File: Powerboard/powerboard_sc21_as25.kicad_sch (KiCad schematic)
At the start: 44 parts, among them J10 Conn_01x04_Male, J2 Conn_01x02_Male, J3 Conn_01x02_Male, J4 Conn_01x08_Male, J9 Conn_Coaxial, Q6 MMDT2222A, Q7 RSJ250P10TL, Q8 RSJ250P10TL, U1 LTC4412xS6, U2 SN65HVD230, U3 ESP32-PICO-D4

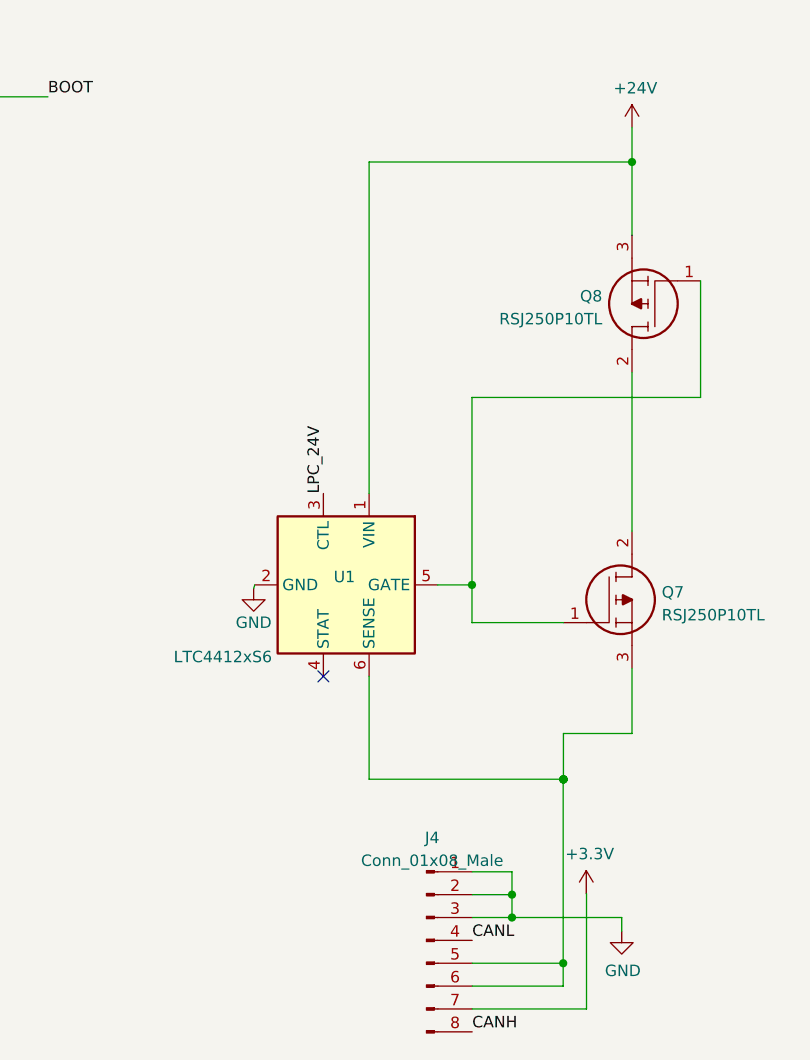
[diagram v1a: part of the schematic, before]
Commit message: update
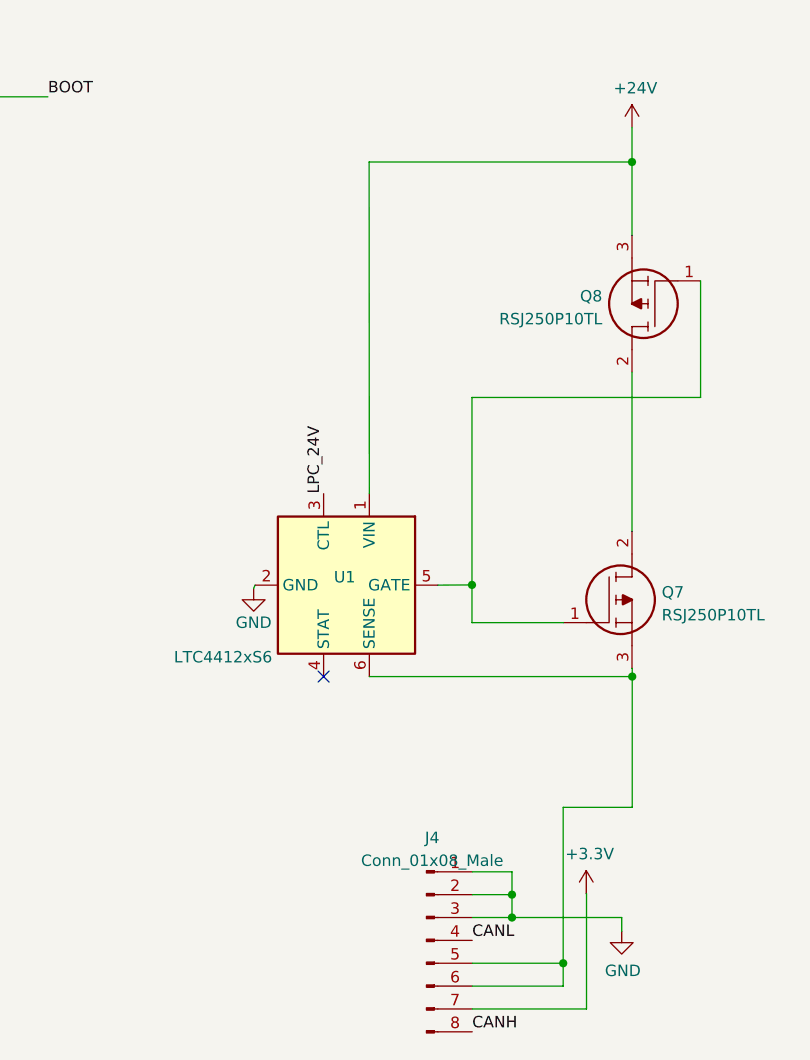
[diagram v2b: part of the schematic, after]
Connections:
- net LPC_24V: no longer U1.3 (CTL)
- net at Q7.3, U1.6 (SENSE): now also J4.5 (Pin_5), J4.6 (Pin_6)
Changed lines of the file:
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@@
   (junction (at 217.17 33.02) (diameter 0) (color 0 0 0 0)
   )
+  (junction (at 150.0124 146.9644) (diameter 0) (color 0 0 0 0)
+  )
   (junction (at 257.81 109.22) (diameter 0) (color 0 0 0 0)
   )
+  (junction (at 52.07 26.67) (diameter 0) (color 0 0 0 0)
+  )
+  (junction (at 109.22 46.99) (diameter 0) (color 0 0 0 0)
+  )
+  (junction (at 52.07 46.99) (diameter 0) (color 0 0 0 0)
+  )
+  (junction (at 243.84 149.86) (diameter 0) (color 0 0 0 0)
+  )
+  (junction (at 132.207 136.779) (diameter 0) (color 0 0 0 0)
+  )
+  (junction (at 136.652 173.736) (diameter 0) (color 0 0 0 0)
+  )
+  (junction (at 48.26 82.55) (diameter 0) (color 0 0 0 0)
+  )
+  (junction (at 236.22 149.86) (diameter 0) (color 0 0 0 0)
+  )
+  (junction (at 136.652 171.196) (diameter 0) (color 0 0 0 0)
+  )
+  (junction (at 212.09 33.02) (diameter 0) (color 0 0 0 0)
+  )
   (junction (at 142.3416 178.816) (diameter 0) (color 0 0 0 0)
   )
-  (junction (at 52.07 26.67) (diameter 0) (color 0 0 0 0)
-  )
-  (junction (at 109.22 46.99) (diameter 0) (color 0 0 0 0)
-  )
-  (junction (at 52.07 46.99) (diameter 0) (color 0 0 0 0)
-  )
-  (junction (at 142.3924 158.3944) (diameter 0) (color 0 0 0 0)
-  )
-  (junction (at 243.84 149.86) (diameter 0) (color 0 0 0 0)
-  )
-  (junction (at 132.207 136.779) (diameter 0) (color 0 0 0 0)
-  )
-  (junction (at 136.652 173.736) (diameter 0) (color 0 0 0 0)
-  )
-  (junction (at 48.26 82.55) (diameter 0) (color 0 0 0 0)
-  )
-  (junction (at 236.22 149.86) (diameter 0) (color 0 0 0 0)
-  )
-  (junction (at 136.652 171.196) (diameter 0) (color 0 0 0 0)
-  )
-  (junction (at 142.367 158.369) (diameter 0) (color 0 0 0 0)
-  )
-  (junction (at 212.09 33.02) (diameter 0) (color 0 0 0 0)
-  )
   (junction (at 99.06 43.18) (diameter 0) (color 0 0 0 0)
   )
@@
   )
   (junction (at 260.35 109.22) (diameter 0) (color 0 0 0 0)
-  )
-  (junction (at 142.3416 158.3944) (diameter 0) (color 0 0 0 0)
   )
   (junction (at 207.01 129.54) (diameter 0) (color 0 0 0 0)
@@
   (no_connect (at 196.85 45.72))
   (no_connect (at 237.49 88.9))
-  (no_connect (at 115.697 146.939))
+  (no_connect (at 115.7224 146.9644))
   (no_connect (at 237.49 60.96))
   (no_connect (at 237.49 76.2))
@@
     (stroke (width 0) (type default) (color 0 0 0 0))
   )
-  (wire (pts (xy 128.397 136.779) (xy 132.207 136.779))
+  (wire (pts (xy 128.4224 136.8044) (xy 132.207 136.779))
     (stroke (width 0) (type default) (color 0 0 0 0))
   )
@@
     (stroke (width 0) (type default) (color 0 0 0 0))
   )
+  (wire (pts (xy 150.0124 161.4932) (xy 142.3416 161.4932))
+    (stroke (width 0) (type default) (color 0 0 0 0))
+  )
   (wire (pts (xy 99.06 40.64) (xy 99.06 43.18))
     (stroke (width 0) (type default) (color 0 0 0 0))
@@
     (stroke (width 0) (type default) (color 0 0 0 0))
   )
+  (wire (pts (xy 150.0124 146.05) (xy 149.987 146.05))
+    (stroke (width 0) (type default) (color 0 0 0 0))
+  )
   (wire (pts (xy 136.652 171.196) (xy 136.652 173.736))
     (stroke (width 0) (type default) (color 0 0 0 0))
@@
     (stroke (width 0) (type default) (color 0 0 0 0))
   )
-  (wire (pts (xy 142.3416 158.3944) (xy 142.3416 178.816))
-    (stroke (width 0) (type default) (color 0 0 0 0))
-  )
   (wire (pts (xy 44.45 26.67) (xy 52.07 26.67))
     (stroke (width 0) (type default) (color 0 0 0 0))
@@
     (stroke (width 0) (type default) (color 0 0 0 0))
   )
-  (wire (pts (xy 149.987 146.05) (xy 149.987 153.289))
-    (stroke (width 0) (type default) (color 0 0 0 0))
-  )
   (wire (pts (xy 214.63 160.02) (xy 214.63 158.75))
     (stroke (width 0) (type default) (color 0 0 0 0))
@@
     (stroke (width 0) (type default) (color 0 0 0 0))
   )
-  (wire (pts (xy 142.367 158.369) (xy 120.777 158.369))
-    (stroke (width 0) (type default) (color 0 0 0 0))
-  )
   (wire (pts (xy 34.29 34.29) (xy 40.64 34.29))
     (stroke (width 0) (type default) (color 0 0 0 0))
@@
     (stroke (width 0) (type default) (color 0 0 0 0))
   )
+  (wire (pts (xy 142.3416 178.816) (xy 142.3416 181.356))
+    (stroke (width 0) (type default) (color 0 0 0 0))
+  )
   (wire (pts (xy 149.987 89.789) (xy 149.987 97.917))
     (stroke (width 0) (type default) (color 0 0 0 0))
@@
     (stroke (width 0) (type default) (color 0 0 0 0))
   )
+  (wire (pts (xy 150.0124 146.9644) (xy 150.0124 161.4932))
+    (stroke (width 0) (type default) (color 0 0 0 0))
+  )
   (wire (pts (xy 243.84 146.05) (xy 243.84 149.86))
     (stroke (width 0) (type default) (color 0 0 0 0))
@@
     (stroke (width 0) (type default) (color 0 0 0 0))
   )
-  (wire (pts (xy 120.777 126.619) (xy 120.777 89.789))
+  (wire (pts (xy 150.0124 146.05) (xy 150.0124 146.9644))
+    (stroke (width 0) (type default) (color 0 0 0 0))
+  )
+  (wire (pts (xy 120.8024 126.6444) (xy 120.777 89.789))
     (stroke (width 0) (type default) (color 0 0 0 0))
   )
@@
     (stroke (width 0) (type default) (color 0 0 0 0))
   )
-  (wire (pts (xy 107.95 137.16) (xy 108.077 136.779))
+  (wire (pts (xy 107.95 137.16) (xy 108.1024 136.8044))
     (stroke (width 0) (type default) (color 0 0 0 0))
   )
@@
     (stroke (width 0) (type default) (color 0 0 0 0))
   )
+  (wire (pts (xy 120.8024 146.9644) (xy 150.0124 146.9644))
+    (stroke (width 0) (type default) (color 0 0 0 0))
+  )
   (wire (pts (xy 226.06 146.05) (xy 226.06 149.86))
     (stroke (width 0) (type default) (color 0 0 0 0))
@@
     (stroke (width 0) (type default) (color 0 0 0 0))
   )
-  (wire (pts (xy 120.777 158.369) (xy 120.777 146.939))
-    (stroke (width 0) (type default) (color 0 0 0 0))
-  )
   (wire (pts (xy 204.47 158.75) (xy 214.63 158.75))
     (stroke (width 0) (type default) (color 0 0 0 0))
@@
     (stroke (width 0) (type default) (color 0 0 0 0))
   )
+  (wire (pts (xy 142.3416 161.4932) (xy 142.3416 178.816))
+    (stroke (width 0) (type default) (color 0 0 0 0))
+  )
   (wire (pts (xy 255.27 158.75) (xy 259.08 158.75))
     (stroke (width 0) (type default) (color 0 0 0 0))
@@
     (stroke (width 0) (type default) (color 0 0 0 0))
   )
-  (wire (pts (xy 142.3924 158.3944) (xy 142.367 158.369))
-    (stroke (width 0) (type default) (color 0 0 0 0))
-  )
   (wire (pts (xy 254 109.22) (xy 257.81 109.22))
     (stroke (width 0) (type default) (color 0 0 0 0))
@@
     (stroke (width 0) (type default) (color 0 0 0 0))
   )
-  (wire (pts (xy 142.3416 178.816) (xy 142.3416 181.356))
-    (stroke (width 0) (type default) (color 0 0 0 0))
-  )
-  (wire (pts (xy 142.367 153.289) (xy 149.987 153.289))
-    (stroke (width 0) (type default) (color 0 0 0 0))
-  )
   (wire (pts (xy 132.207 136.779) (xy 132.207 140.97))
-    (stroke (width 0) (type default) (color 0 0 0 0))
-  )
-  (wire (pts (xy 142.367 153.289) (xy 142.367 158.369))
     (stroke (width 0) (type default) (color 0 0 0 0))
   )
@@
     (pin "1")
   )
-  (symbol (lib_id "Power_Management:LTC4412xS6") (at 118.237 136.779 270) (unit 1)
-    (in_bom yes) (on_board yes)
-    (property "Reference" "U1" (id 0) (at 116.84 135.89 90)
-      (effects (font (size 1.27 1.27)) (justify left))
-    )
-    (property "Value" "LTC4412xS6" (id 1) (at 99.06 144.78 90)
-      (effects (font (size 1.27 1.27)) (justify left))
-    )
-    (property "Footprint" "Package_TO_SOT_SMD:TSOT-23-6" (id 2) (at 109.347 153.289 0)
-      (effects (font (size 1.27 1.27)) hide)
-    )
-    (property "Datasheet" "https://www.analog.com/media/en/technical-documentation/data-sheets/4412fb.pdf" (id 3) (at 113.157 190.119 0)
-      (effects (font (size 1.27 1.27)) hide)
-    )
+  (symbol (lib_id "Power_Management:LTC4412xS6") (at 118.2624 136.8044 270) (unit 1)
+    (in_bom yes) (on_board yes)
+    (property "Reference" "U1" (id 0) (at 116.8654 135.9154 90)
+      (effects (font (size 1.27 1.27)) (justify left))
+    )
+    (property "Value" "LTC4412xS6" (id 1) (at 99.0854 144.8054 90)
+      (effects (font (size 1.27 1.27)) (justify left))
+    )
+    (property "Footprint" "Package_TO_SOT_SMD:TSOT-23-6" (id 2) (at 109.3724 153.3144 0)
+      (effects (font (size 1.27 1.27)) hide)
+    )
+    (property "Datasheet" "https://www.analog.com/media/en/technical-documentation/data-sheets/4412fb.pdf" (id 3) (at 113.1824 190.1444 0)
+      (effects (font (size 1.27 1.27)) hide)
+    )
